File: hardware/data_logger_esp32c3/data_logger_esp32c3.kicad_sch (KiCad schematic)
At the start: 51 parts, among them U1 ESP32-C3-MINI-1, U2 MC34063ADRJR, U3 LM321MF, U4 LM321MF, U5 LM321MF, U6 LM321MF, U7 LM321MF, U8 LM321MF

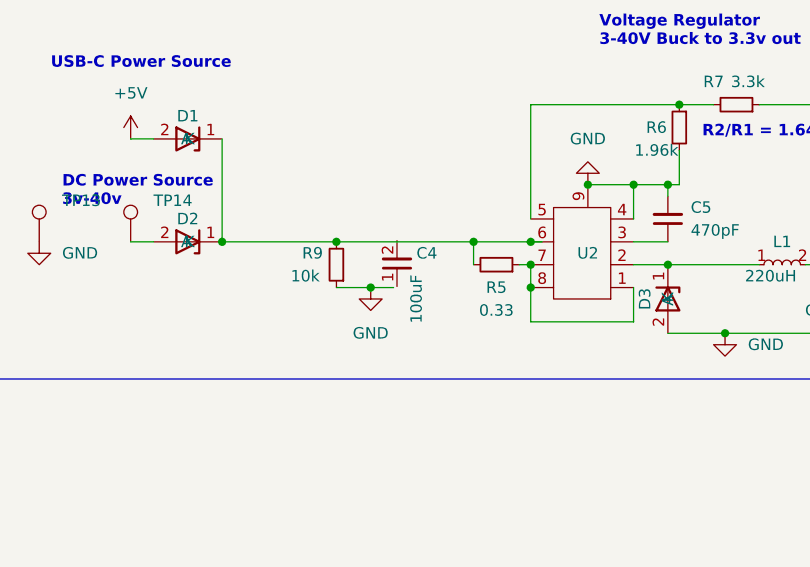
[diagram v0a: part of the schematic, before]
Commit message: last commit of the night
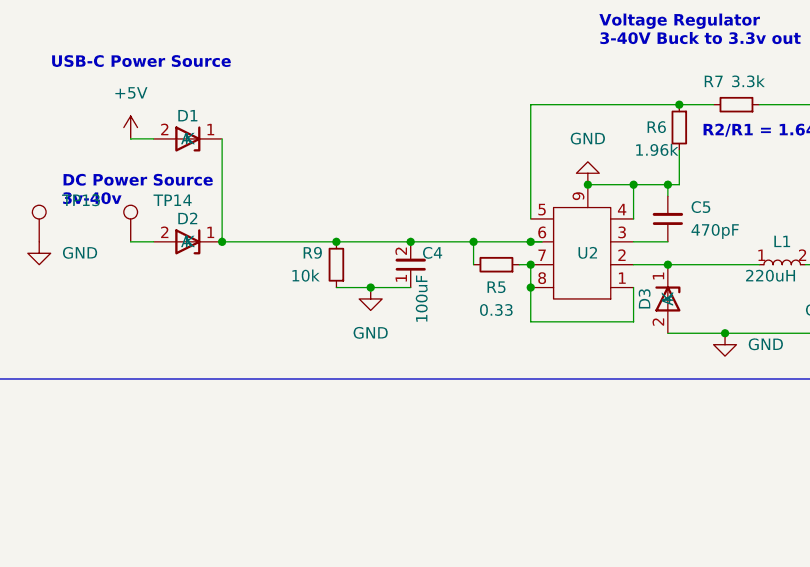
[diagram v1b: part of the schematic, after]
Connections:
- net GND: now also C4.1
- net at C4.2: now also D1.1 (K), D2.1 (K), R5.2, R9.2, U2.6 (Vcc)
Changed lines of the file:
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@@
   (junction (at 302.26 181.61) (diameter 0) (color 0 0 0 0)
+  )
+  (junction (at 81.915 270.51) (diameter 0) (color 0 0 0 0)
   )
   (junction (at 300.99 113.03) (diameter 0) (color 0 0 0 0)
@@
     (stroke (width 0) (type default) (color 0 0 0 0))
   )
-  (wire (pts (xy 77.47 275.59) (xy 80.01 275.59))
+  (wire (pts (xy 77.47 275.59) (xy 81.915 275.59))
     (stroke (width 0) (type default) (color 0 0 0 0))
   )
@@
     (stroke (width 0) (type default) (color 0 0 0 0))
   )
-  (wire (pts (xy 73.66 270.51) (xy 88.9 270.51))
-    (stroke (width 0) (type default) (color 0 0 0 0))
-  )
   (wire (pts (xy 312.42 57.15) (xy 314.96 57.15))
     (stroke (width 0) (type default) (color 0 0 0 0))
@@
     (stroke (width 0) (type default) (color 0 0 0 0))
   )
+  (wire (pts (xy 81.915 270.51) (xy 88.9 270.51))
+    (stroke (width 0) (type default) (color 0 0 0 0))
+  )
   (wire (pts (xy 261.62 281.94) (xy 288.29 281.94))
     (stroke (width 0) (type default) (color 0 0 0 0))
@@
   )
   (wire (pts (xy 111.76 260.35) (xy 111.76 264.16))
+    (stroke (width 0) (type default) (color 0 0 0 0))
+  )
+  (wire (pts (xy 73.66 270.51) (xy 81.915 270.51))
     (stroke (width 0) (type default) (color 0 0 0 0))
   )
@@
     (pin "4")
     (pin "5")
-  )
-  (symbol (lib_id "lib:RT1H101M0810") (at 76.2 273.05 90) (unit 1)
-    (in_bom yes) (on_board yes)
-    (property "Reference" "C4" (id 0) (at 82.55 271.78 90)
-      (effects (font (size 1.27 1.27)) (justify right))
-    )
-    (property "Value" "100uF" (id 1) (at 82.55 276.86 0))
-    (property "Footprint" "lib:RT1H101M0810" (id 2) (at 76.2 273.05 0)
-      (effects (font (size 1.27 1.27)) hide)
-    )
-    (property "Datasheet" "" (id 3) (at 76.2 273.05 0)
-      (effects (font (size 1.27 1.27)) hide)
-    )
-    (property "part_number" "RT1H101M0810" (id 4) (at 83.82 274.1865 90)
-      (effects (font (size 1.27 1.27)) (justify right) hide)
-    )
-    (pin "1")
-    (pin "2")
   )
   (symbol (lib_id "Connector:TestPoint") (at 88.9 101.6 0) (unit 1)
@@
     (pin "1")
   )
+  (symbol (lib_id "lib:RT1H101M0810") (at 76.835 273.05 90) (unit 1)
+    (in_bom yes) (on_board yes)
+    (property "Reference" "C4" (id 0) (at 83.185 271.78 90)
+      (effects (font (size 1.27 1.27)) (justify right))
+    )
+    (property "Value" "100uF" (id 1) (at 83.185 276.86 0))
+    (property "Footprint" "lib:RT1H101M0810" (id 2) (at 76.835 273.05 0)
+      (effects (font (size 1.27 1.27)) hide)
+    )
+    (property "Datasheet" "" (id 3) (at 76.835 273.05 0)
+      (effects (font (size 1.27 1.27)) hide)
+    )
+    (property "part_number" "RT1H101M0810" (id 4) (at 84.455 274.1865 90)
+      (effects (font (size 1.27 1.27)) (justify right) hide)
+    )
+    (pin "1")
+    (pin "2")
+  )
   (symbol (lib_id "Device:C_Small") (at 110.49 267.97 180) (unit 1)
     (in_bom yes) (on_board yes) (fields_autoplaced)
@@
       (reference "C3") (unit 1) (value "0.1uF") (footprint "Capacitor_SMD:C_0603_1608Metric")
     )
-    (path "/2655c89d-2a06-4196-8ce2-d0090623db72"
+    (path "/e6638ff8-c3a0-4480-81b5-384e94fa18a7"
       (reference "C4") (unit 1) (value "100uF") (footprint "lib:RT1H101M0810")
     )
